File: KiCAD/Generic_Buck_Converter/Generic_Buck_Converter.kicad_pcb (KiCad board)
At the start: 4 copper layers, 17.8 x 27 mm, 20 parts, among them IC1 MAX17634C, J1 Conn_01x05

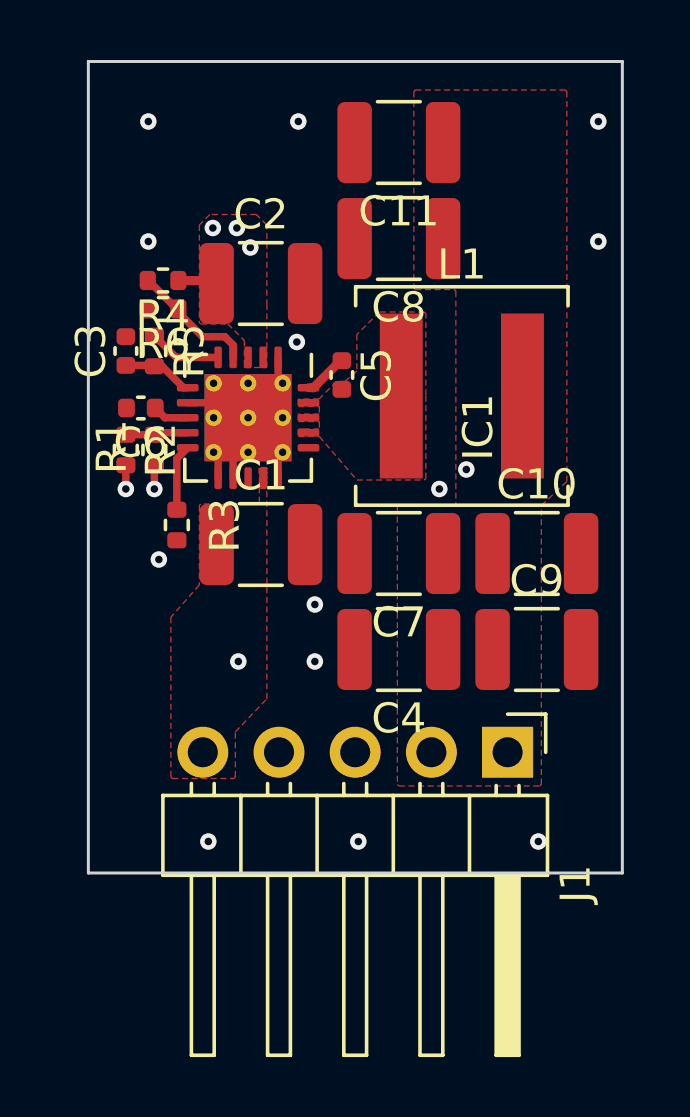
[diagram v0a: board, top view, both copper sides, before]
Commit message: Schematic orderlist update
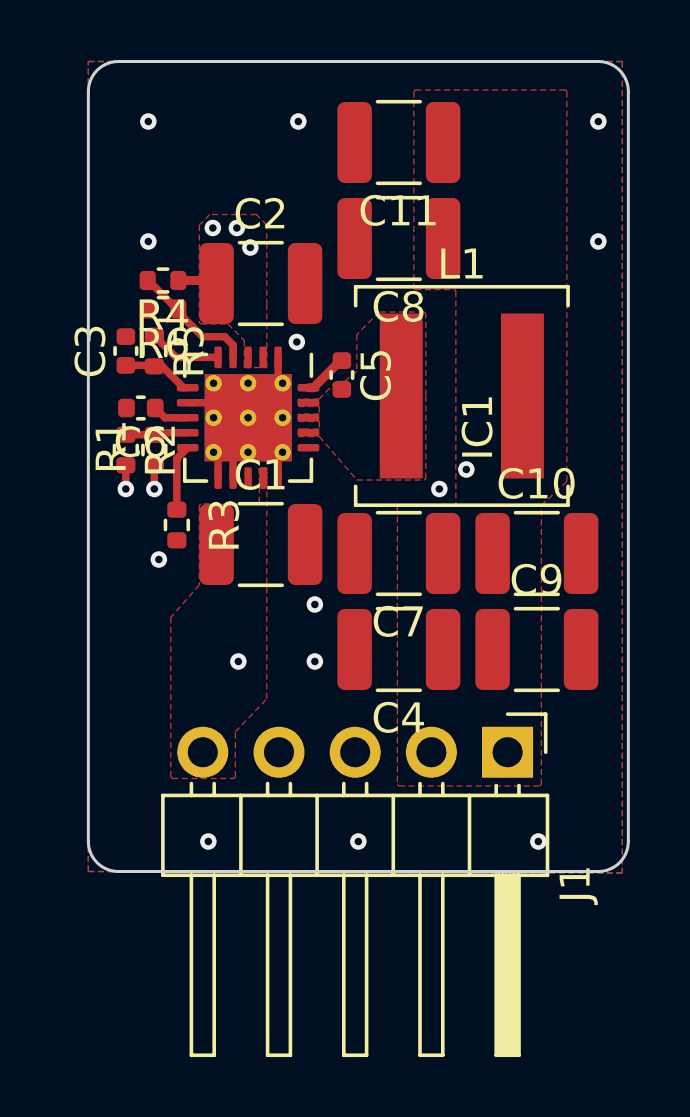
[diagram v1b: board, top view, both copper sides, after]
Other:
- board size 17.8 x 27 mm -> 18 x 27 mm
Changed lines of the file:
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@@
     )
   )
-  (gr_rect (start 100 100) (end 117.8 127.05)
-    (stroke (width 0.1) (type default)) (fill none) (layer "Edge.Cuts"))
+  (gr_arc (start 100 101) (mid 100.292893 100.292893) (end 101 100)
+    (stroke (width 0.1) (type default)) (layer "Edge.Cuts"))
+  (gr_arc (start 117 100) (mid 117.707107 100.292893) (end 118 101)
+    (stroke (width 0.1) (type default)) (layer "Edge.Cuts"))
+  (gr_line (start 101 127) (end 117 127)
+    (stroke (width 0.1) (type default)) (layer "Edge.Cuts"))
+  (gr_arc (start 101 127) (mid 100.292893 126.707107) (end 100 126)
+    (stroke (width 0.1) (type default)) (layer "Edge.Cuts"))
+  (gr_arc (start 118 126) (mid 117.707107 126.707107) (end 117 127)
+    (stroke (width 0.1) (type default)) (layer "Edge.Cuts"))
+  (gr_line (start 118 126) (end 118 101)
+    (stroke (width 0.1) (type default)) (layer "Edge.Cuts"))
+  (gr_line (start 117 100) (end 101 100)
+    (stroke (width 0.1) (type default)) (layer "Edge.Cuts"))
+  (gr_line (start 100 101) (end 100 126)
+    (stroke (width 0.1) (type default)) (layer "Edge.Cuts"))
   (gr_text "JLCJLCJLCJLC" (at 108.55 101.35) (layer "B.SilkS")
     (effects (font (size 0.8 0.8) (thickness 0.15) bold) (justify left bottom mirror))
@@
         (xy 105.95 121.245244)
         (xy 105.95 113.55)
-        (xy 105.95 113.55)
         (xy 105.7 113.55)
         (xy 105.7 113.8)
@@
         (xy 117.8 100)
         (xy 117.8 127.05)
-        (xy 100 127.05)
-      )
-    )
+        (xy 100 127)
+      )
+    )
